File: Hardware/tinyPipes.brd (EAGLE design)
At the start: 59 x 59 mm, 109 parts, among them J1 Micro-USB connector, Q1 CJ2302, Q2 BSS84, Q5 S9013, Q6 S9013, Q7 S9013, Q8 BSS123, Q9 BSS123, U1 TD1410, U2 ICS_V54_SIM900, U3 ATMEGA168, U4 MAX4372, U5 SI4435POWER

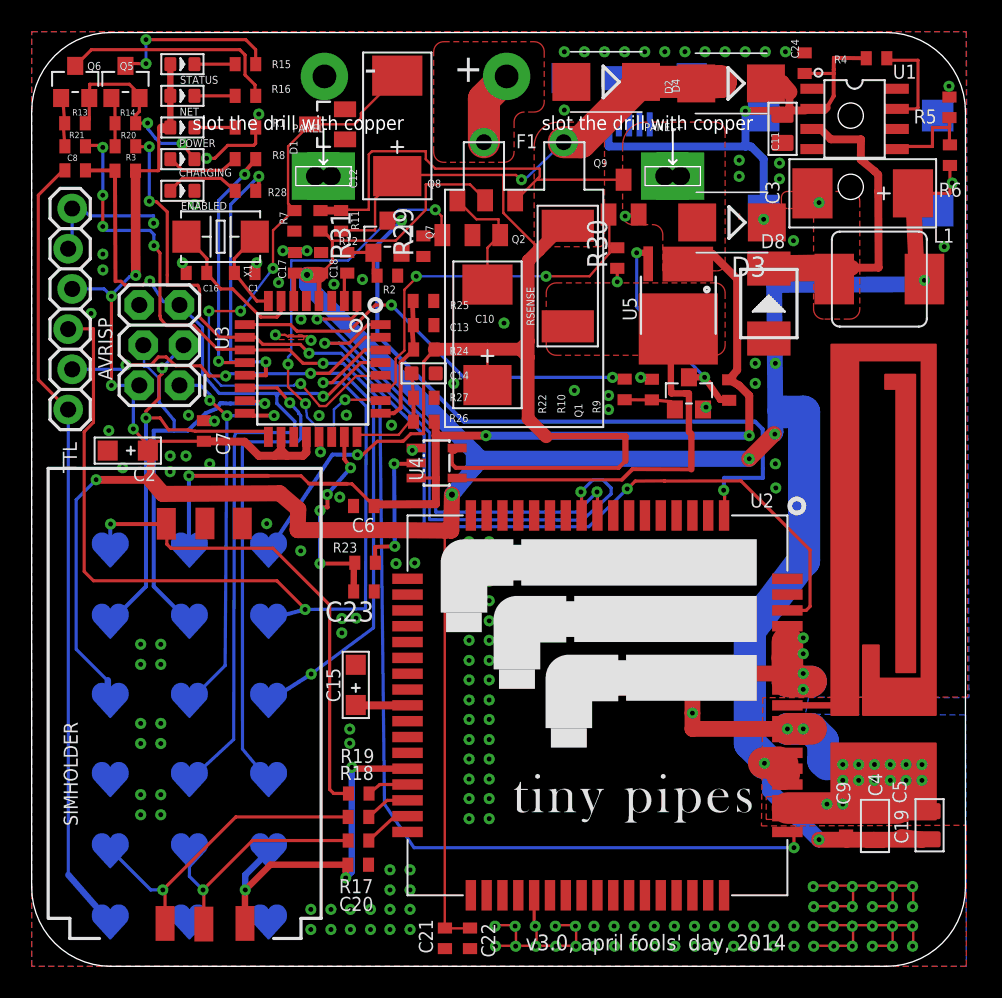
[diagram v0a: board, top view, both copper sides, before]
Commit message: tinyPipes v3.1
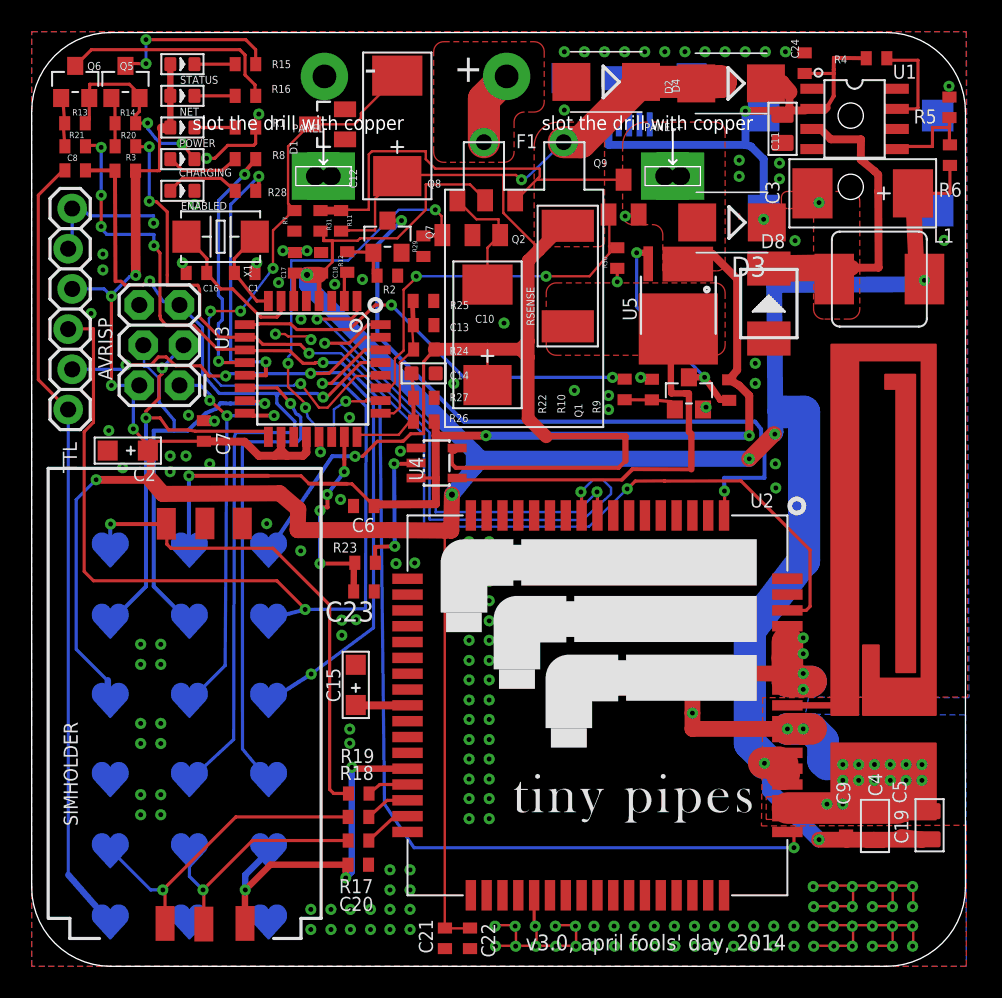
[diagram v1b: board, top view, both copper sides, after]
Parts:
- R11: value (none) -> 10k
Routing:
- net GND: vias 215 -> 211
